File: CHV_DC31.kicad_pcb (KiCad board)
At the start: 2 copper layers, 137.3 x 128.4 mm, 103 parts, among them IC1 W25Q16JVUXIQ_TR, J1 USB_C_Receptacle_USB2.0, J2 Conn_01x02, J3 Conn_02x03_Odd_Even, J4 Conn_02x03_Odd_Even, J5 Conn_02x03_Odd_Even, J6 Conn_01x03, Q1 PMOS, U1 MCP2558FD-xMNY, U2 XC6220B331MR, U3 RP2040, U4 MCP2558FD-xMNY, U5 MCP2558FD-xMNY, U6 MCP2558FD-xMNY, U7 HT75xx-1-SOT89, Y1 XYDBPCNANF-12MHz

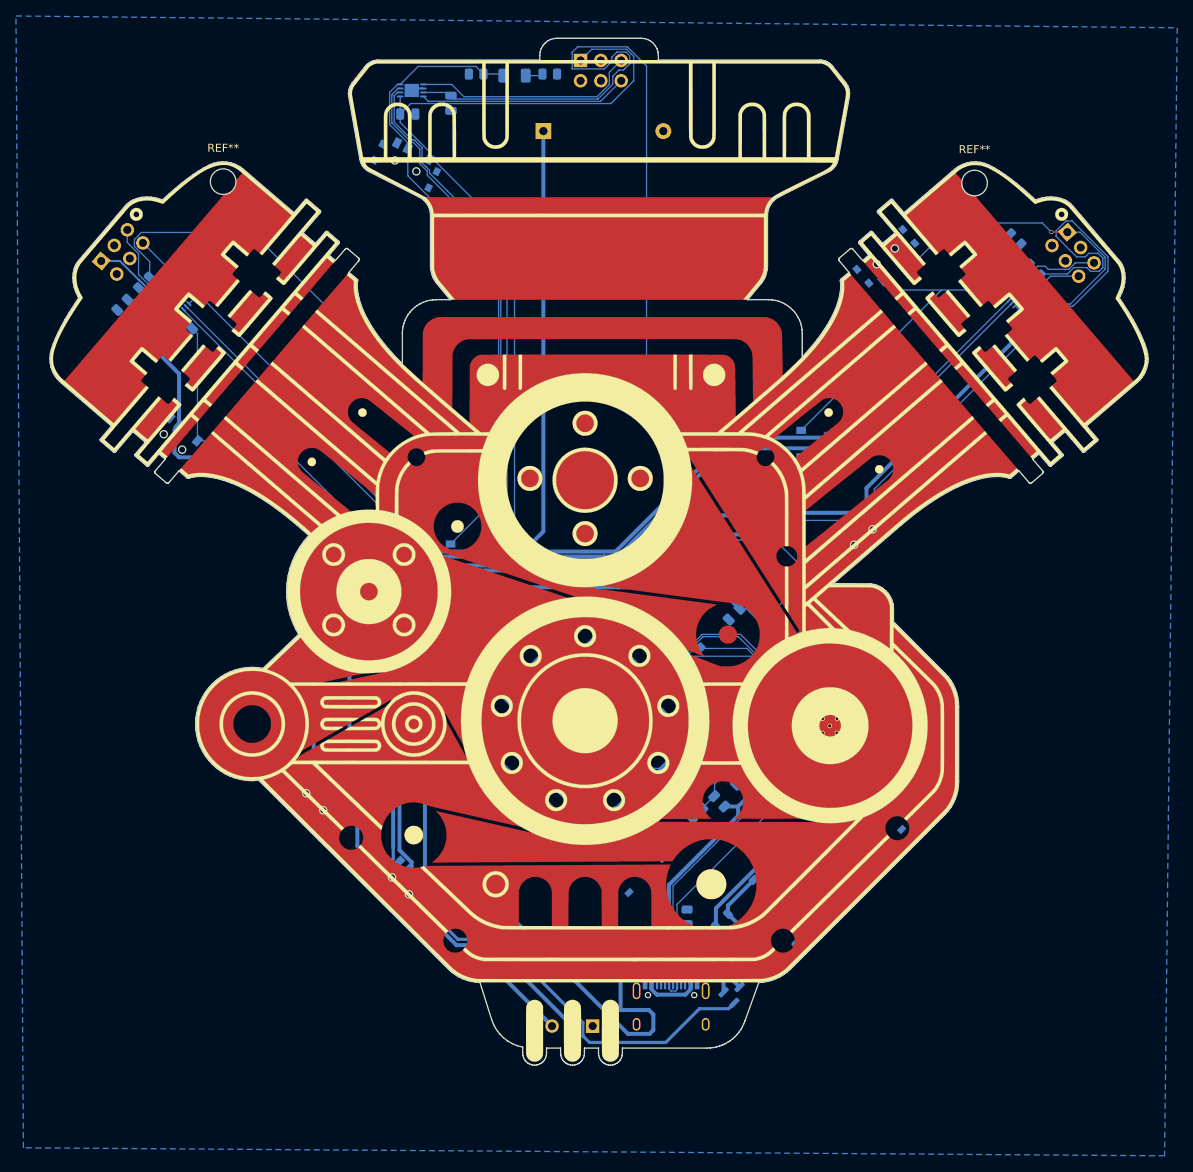
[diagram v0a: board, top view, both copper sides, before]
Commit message: We are SOOOOO close
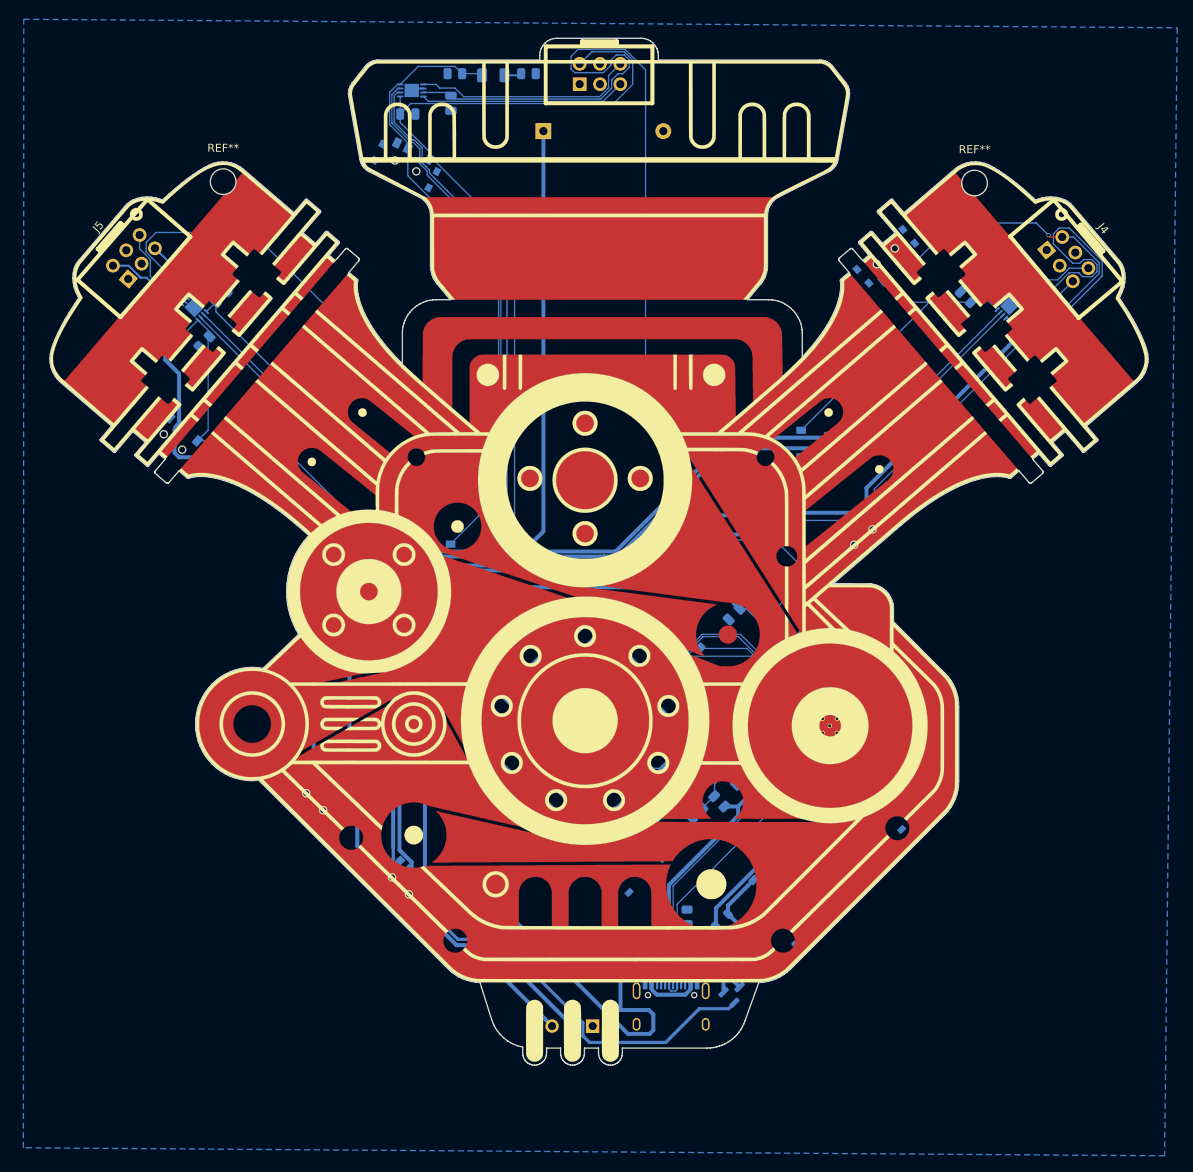
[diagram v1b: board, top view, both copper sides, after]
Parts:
- J3, J4, J5: footprint Connector_PinHeader_2.54mm:PinHeader_2x03_P2.54mm_Vertical -> badgelife_sao_v169bis:Badgelife-SAOv169-BADGE-2x3; moved to F.Cu
- moved J5 4.07 mm to (69.9, 56.7), turned to 49 degrees
- moved J4 3.31 mm to (186.6, 56.9), turned to -50 degrees
- moved J3 2.90 mm to (128.2, 33.8), turned to 0 degrees
- moved R17 2.66 mm to (119.3, 33.8)
- moved D10 2.66 mm to (114.9, 34.0)
- moved R18 2.66 mm to (110.1, 33.8)
- moved R22 2.40 mm to (78.8, 67.3)
- moved C24 2.40 mm to (80.9, 61.7)
- moved U6 2.40 mm to (77.5, 63.0)
- moved D14 2.40 mm to (74.8, 65.5)
- moved C23 2.40 mm to (73.5, 60.9)
- moved R21 2.40 mm to (70.7, 63.7)
- moved C21 1.91 mm to (181.3, 59.9)
- moved R19 1.91 mm to (179.0, 56.0)
- moved R20 1.91 mm to (174.0, 61.7)
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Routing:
- net +3V3: track 641.6 -> 638.0 mm
- net Net-(J6-Pin_2): track 299.0 -> 295.5 mm
- net Net-(J6-Pin_3): track 300.1 -> 296.7 mm
- net Net-(D10-A): track 80.6 -> 78.0 mm
- net Net-(D11-K): track 42.1 -> 39.4 mm
- net VBUS: track 413.6 -> 411.6 mm
- net Net-(D13-K): track 52.9 -> 51.8 mm
- net SAO2_RX: track 6.60 -> 7.39 mm
- net SAO3_RX: track 7.08 -> 7.73 mm
- net Net-(D12-K): track 2.90 -> 2.27 mm
- net SAO3_TX: track 10.4 -> 11.1 mm
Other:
- board text added: "Silent"
